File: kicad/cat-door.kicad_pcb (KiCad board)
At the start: 2 copper layers, 25 x 48.6 mm, 18 parts, among them U1 ATtiny84-20PU, U2 L293D, U3 LF50_TO220

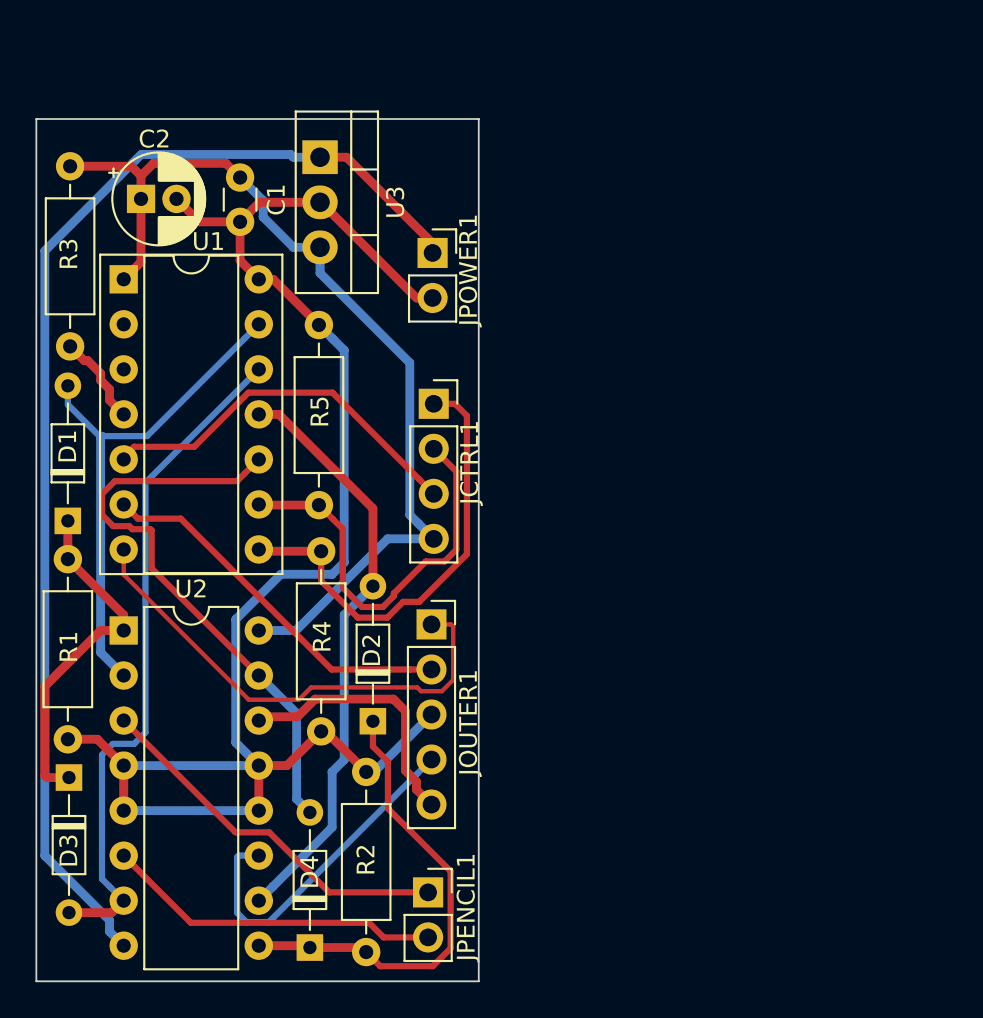
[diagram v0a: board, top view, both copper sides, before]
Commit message: PCB seems done
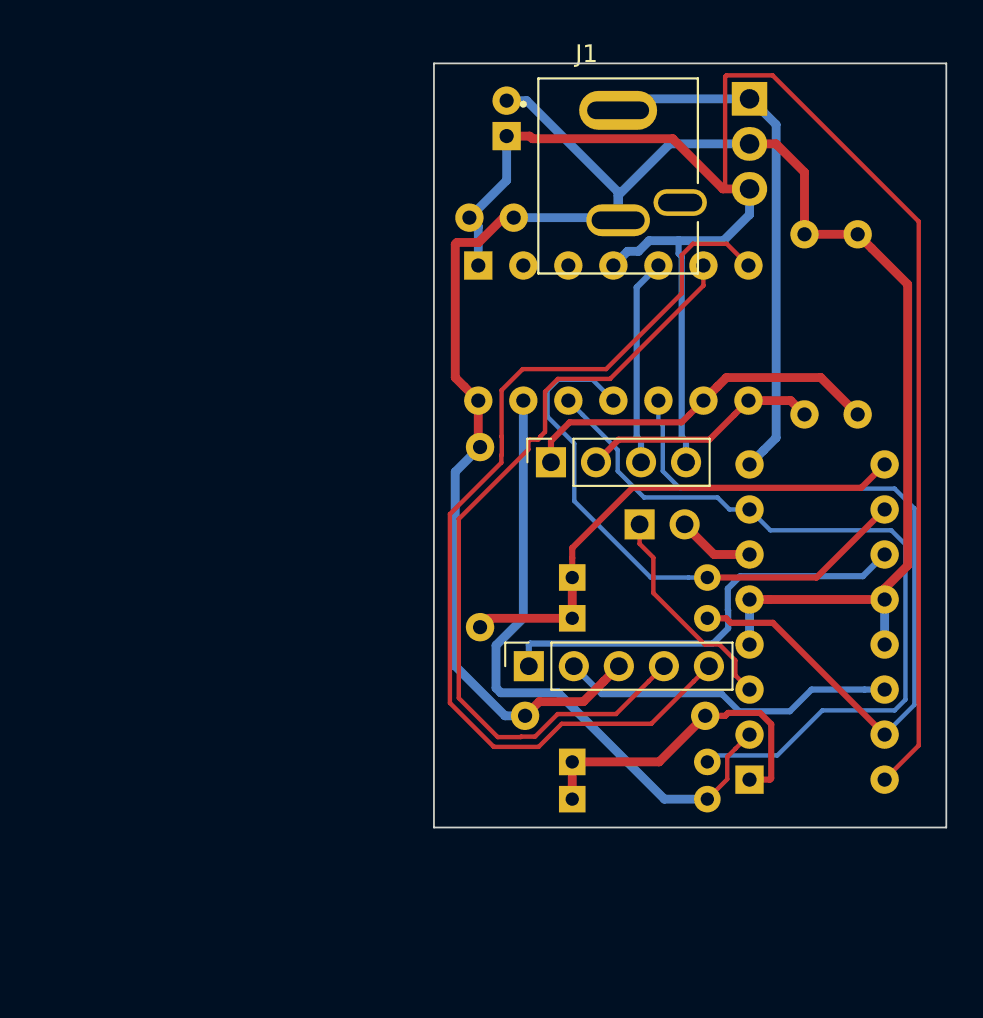
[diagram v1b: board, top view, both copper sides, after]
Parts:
- removed JPOWER1: Conn_01x02, Connector_PinSocket_2.54mm:PinSocket_1x02_P2.54mm_Vertical
- removed R3: 10k, Resistor_THT:R_Axial_DIN0207_L6.3mm_D2.5mm_P10.16mm_Horizontal
- added G***: LOGO, Cat Door:cat, B.Cu at (85.2, 39.8)
- added J1: Barrel_Jack_Switch, Cat Door:CUI_PJ-044AH, F.Cu at (71.5, 41.9)
- C1, C2, D1, D2, D3, D4, JPENCIL1, R1, R2, R4, R5, U1, U2, U3: moved to B.Cu
- moved R1 37.0 mm to (76.4, 72.4), turned to 180 degrees
- moved U2 36.3 mm to (78.9, 76.0)
- moved D1 32.5 mm to (68.9, 77.1), turned to 0 degrees
- moved R4 31.2 mm to (85.0, 55.4), turned to 90 degrees
- moved D3 28.4 mm to (68.9, 75.0), turned to 0 degrees
- moved R5 27.9 mm to (82.0, 55.4)
- moved U3 24.4 mm to (78.9, 37.6)
- moved JPENCIL1 23.9 mm to (72.7, 61.6), turned to 270 degrees
- moved D4 23.7 mm to (68.9, 66.9), turned to 0 degrees
- moved C2 20.9 mm to (65.2, 39.7), turned to 90 degrees
- moved U1 20.0 mm to (63.6, 47.0), turned to 270 degrees
- moved R2 19.4 mm to (63.7, 67.4)
- moved D2 13.9 mm to (68.9, 64.6), turned to 0 degrees
- moved C1 13.1 mm to (63.1, 44.3), turned to 0 degrees
- moved JCTRL1 7.39 mm to (67.7, 58.1), turned to 90 degrees
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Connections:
- JCTRL1 pad 1: /sw_closed_i -> /sw_open_i
- JCTRL1 pad 2: /sw_open_i -> /sw_closed_i
- JOUTER1 pad 1: /sens_open_i -> Net-(JOUTER1-Pad1)
- JOUTER1 pad 2: /sens_closed_i -> Net-(JOUTER1-Pad2)
- JOUTER1 pad 4: Net-(JOUTER1-Pad4) -> /sens_closed_i
- JOUTER1 pad 5: Net-(JOUTER1-Pad5) -> /sens_open_i
- R4 pad 1: /sw_closed_i -> /sw_open_i
- R5 pad 1: /sw_open_i -> /sw_closed_i
- U1 pad 4: Net-(R3-Pad2) -> +5V
- U2 pad 11: Net-(JOUTER1-Pad4) -> Net-(JOUTER1-Pad1)
- U2 pad 14: Net-(JOUTER1-Pad5) -> Net-(JOUTER1-Pad2)
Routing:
- net +5V: track 54.5 -> 100.6 mm
- net +9V: track 67.8 -> 29.6 mm
- net /sens_open_i: track 27.8 -> 55.5 mm
- net /sens_closed_i: track 21.2 -> 46.3 mm
- net Net-(JOUTER1-Pad1): track 0.00 -> 24.7 mm
- net Net-(JOUTER1-Pad4): track 19.4 -> 0.00 mm
- net Net-(JOUTER1-Pad2): track 0.00 -> 19.1 mm
- net GND: track 92.9 -> 111.8 mm
- net Net-(JOUTER1-Pad5): track 14.9 -> 0.00 mm
- net Net-(JPENCIL1-Pad2): track 19.1 -> 4.39 mm
- net /sw_closed_i: track 25.8 -> 13.5 mm
- net /outer_down_o: track 33.6 -> 45.3 mm
- net /flshgnd: track 21.5 -> 11.7 mm
- net Net-(JPENCIL1-Pad1): track 21.2 -> 12.4 mm
- net /inner_up_o: track 29.3 -> 36.0 mm
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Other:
- board size 25 x 48.6 mm -> 28.9 x 43.1 mm
- board text added: "Mark's Cat Door Rev. 2"
